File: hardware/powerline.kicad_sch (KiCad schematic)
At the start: 13 parts, among them J1 Terminal_1x2, J2 Terminal_1x4, Q1 BTA316B-800E, U1 ESP32-WROOM-32E, U2 MOC3063S

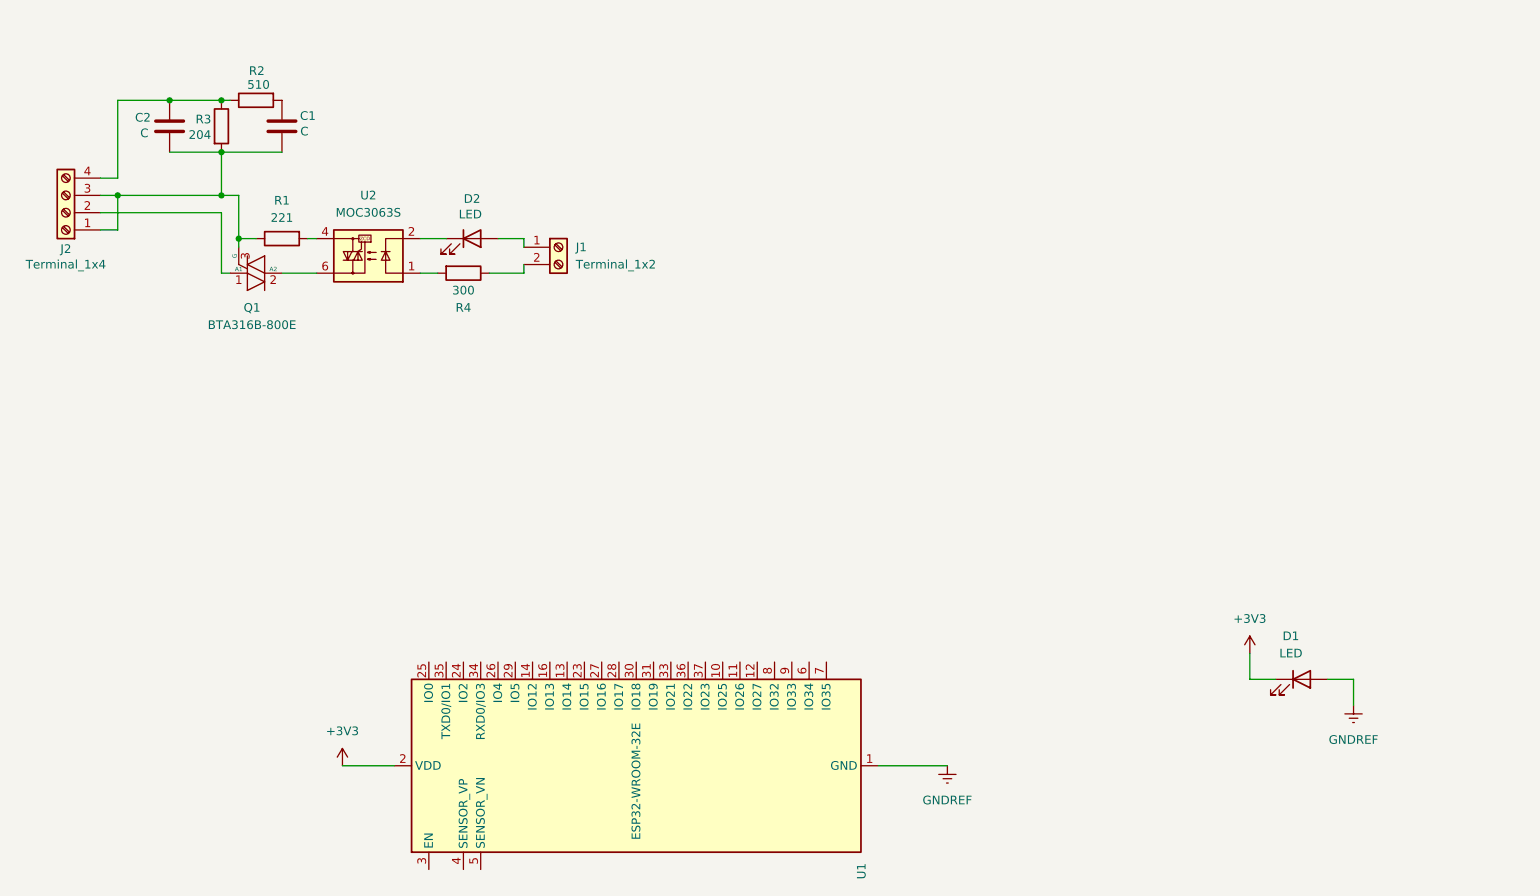
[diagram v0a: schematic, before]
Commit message: add power feed
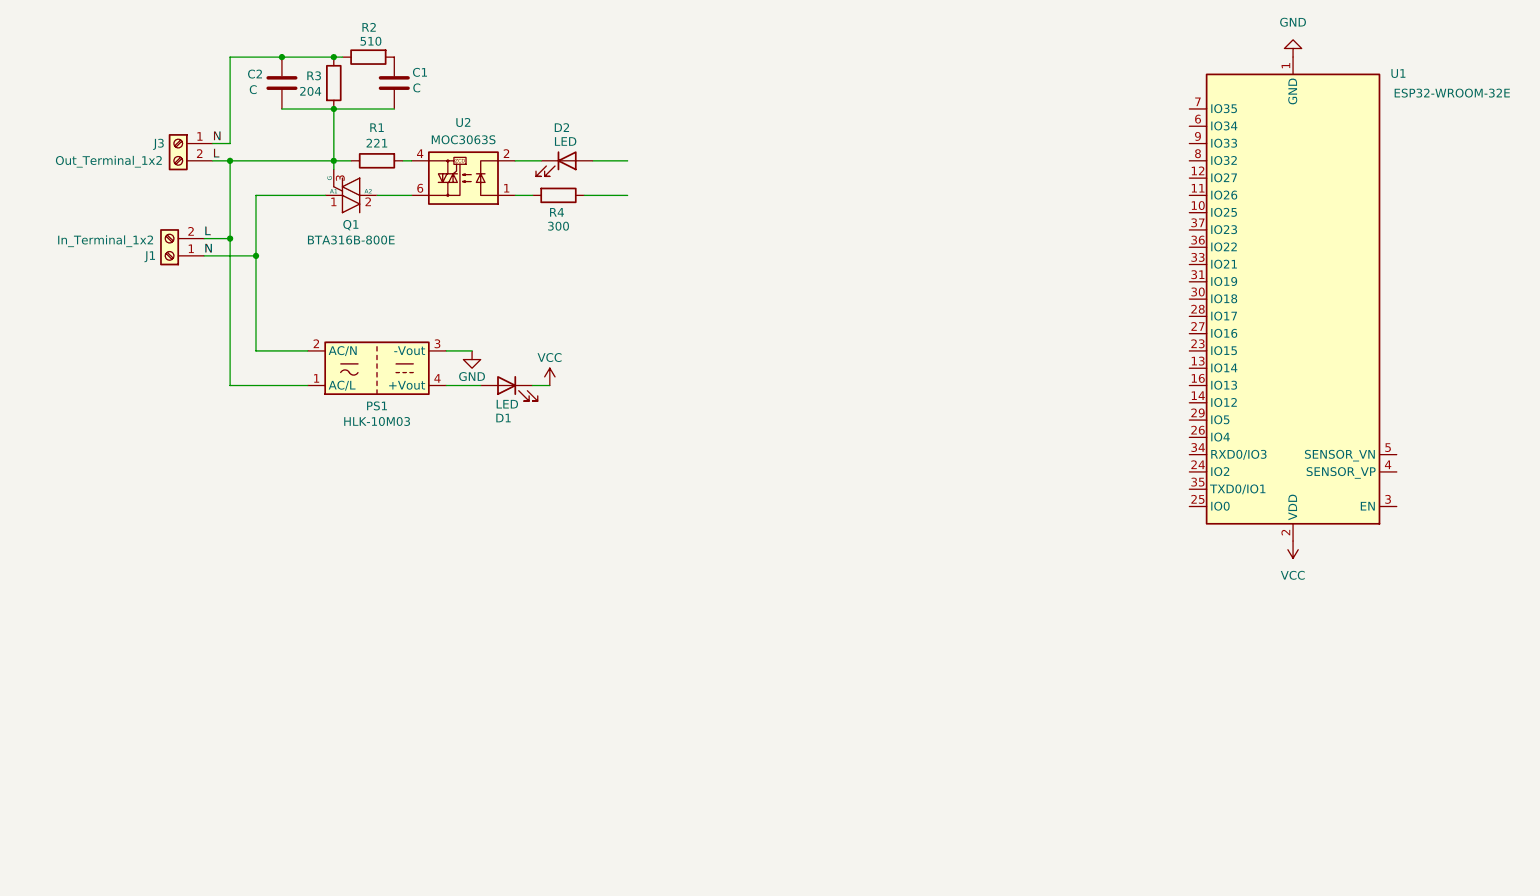
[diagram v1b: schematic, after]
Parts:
- removed J2: Terminal_1x4, symbol Connector:Screw_Terminal_01x04
- added J3: Out_Terminal_1x2, symbol Connector:Screw_Terminal_01x02
- added PS1: HLK-10M03, Converter_ACDC:Converter_ACDC_Hi-Link_HLK-10Mxx, symbol Converter_ACDC:HLK-10M03
- J1: value Terminal_1x2 -> In_Terminal_1x2
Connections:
- net N: now reaches Q1.1 (A1)
- net N: now also C2.1, J1.1 (Pin_1), R2.1, R3.1, J3.1 (Pin_1), PS1.2 (AC/N)
- net L: now reaches C1.2, C2.2, Q1.3 (G), R1.1, R3.2
- net L: now also J1.2 (Pin_2), J3.2 (Pin_2), PS1.1 (AC/L)
- net at D2.2 (A): no longer J1.1 (Pin_1)
- net at R4.1: no longer J1.2 (Pin_2)
- net +3V3 renamed VCC
- net GNDREF renamed GND
- net GND: now also PS1.3 (-Vout); no longer D1.2 (A)
- new net: D1.2 (A), PS1.4 (+Vout)
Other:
- moved on the sheet: C1, C2, D1, D2, J1, Q1, R1, R2, R3, R4, U1, U2
